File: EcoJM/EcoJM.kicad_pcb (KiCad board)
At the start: 2 copper layers, 49.2 x 99 mm, 50 parts, among them J1 Conn_01x01_Pin, J10 Conn_01x01_Pin, J11 Conn_01x01_Pin, J2 Conn_01x01_Pin, J3 Conn_01x02_Pin, J4 Conn_01x02_Pin, J5 Conn_01x03_Pin, J6 Conn_01x02_Pin, J7 Conn_01x03_Pin, J8 Screw_Terminal_01x02, J9 Screw_Terminal_01x02, Q1 2SD882_C842818, Q2 2SD882_C842818, U1 ACS712xLCTR-30A, U2 MT2492, U3 SIT65HVD230DR, U4 AZ1117-3.3, U5 RS321BXF, U6 STM32F_dev, U7 PC817C_C3025164, U8 PC817C_C3025164

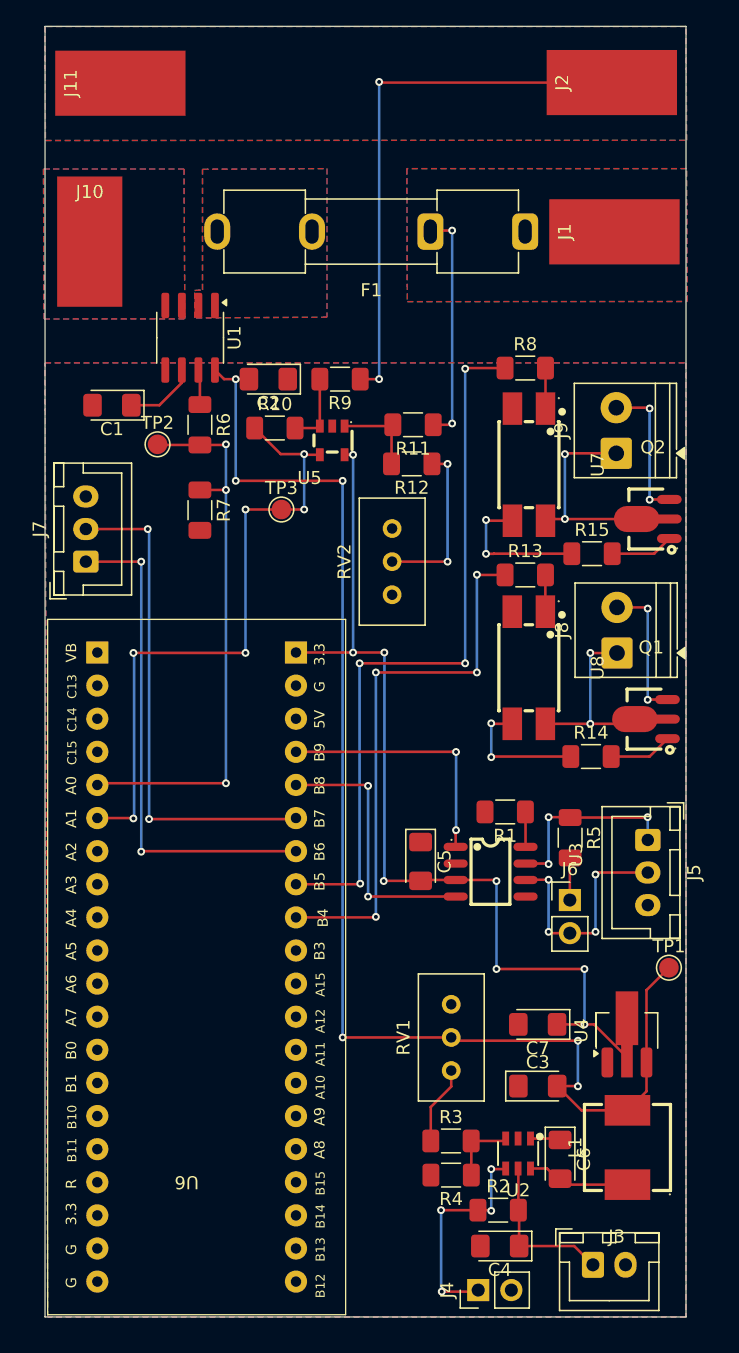
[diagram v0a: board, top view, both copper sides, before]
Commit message: RevA finito, revision, reroute, refurbish
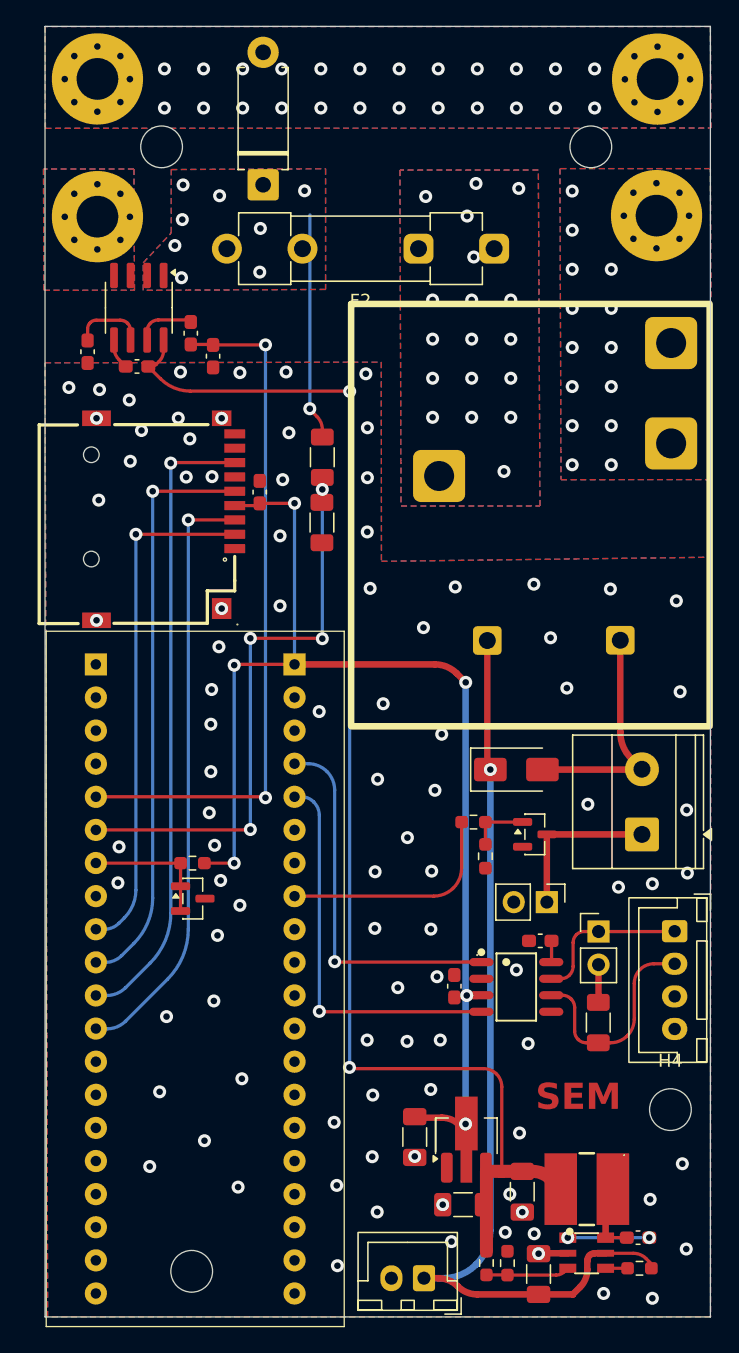
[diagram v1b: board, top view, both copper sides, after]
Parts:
- removed C3, C4: 22u, LED_SMD:LED_1206_3216Metric_Pad1.42x1.75mm_HandSolder
- removed C6: 22n, LED_SMD:LED_1206_3216Metric_Pad1.42x1.75mm_HandSolder
- removed F1: Fuse, Fuse:Fuseholder_Clip-5x20mm_Keystone_3512_Inline_P23.62x7.27mm_D1.02x1.57mm_Horizontal
- removed J11, J2: Conn_01x01_Pin, Connector_Wire:SolderWirePad_1x01_SMD_5x10mm
- removed L1: 10u, EasyEDA:IND-SMD_L7.2-W6.6_GPSR07X0
- removed Q2: 2SD882_C842818, EasyEDA:SOT-89-3_L4.5-W2.5-P1.50-LS4.1-BR
- removed R1, R2, R4: 10k, Resistor_SMD:R_1206_3216Metric_Pad1.30x1.75mm_HandSolder
- removed R13, R8: 470, Resistor_SMD:R_1206_3216Metric_Pad1.30x1.75mm_HandSolder
- removed R14, R15: 100, Resistor_SMD:R_1206_3216Metric_Pad1.30x1.75mm_HandSolder
- removed R3: 68k, Resistor_SMD:R_1206_3216Metric_Pad1.30x1.75mm_HandSolder
- removed R5: 120, Resistor_SMD:R_1206_3216Metric_Pad1.30x1.75mm_HandSolder
- removed RV1, RV2: 10k, Potentiometer_THT:Potentiometer_Bourns_3296W_Vertical
- removed TP1, TP2, TP3: TestPoint, TestPoint:TestPoint_Pad_D1.5mm
- removed U3: SIT65HVD230DR, EasyEDA:SOP-8_L4.9-W3.9-P1.27-LS6.0-BL
- removed U7, U8: PC817C_C3025164, EasyEDA:OPTO-SMD-4_L4.6-W6.5-P2.54-LS10.3-TL
- added C10: 10u, Capacitor_SMD:C_1206_3216Metric_Pad1.33x1.80mm_HandSolder, F.Cu at (103.2, 141.6)
- added C11: 22u, Capacitor_SMD:C_1206_3216Metric_Pad1.33x1.80mm_HandSolder, F.Cu at (97.4, 136.3)
- added C8: 1u, Capacitor_SMD:C_0603_1608Metric_Pad1.08x0.95mm_HandSolder, F.Cu at (81.8, 81.7)
- added C9: 22n, Capacitor_SMD:C_0603_1608Metric_Pad1.08x0.95mm_HandSolder, F.Cu at (110.9, 138.9)
- added C9: 22u, Capacitor_SMD:C_1206_3216Metric_Pad1.33x1.80mm_HandSolder, F.Cu at (102.0, 135.3)
- added D1: P6KE47A, Diode_THT:D_DO-15_P10.16mm_Horizontal, F.Cu at (82.1, 58.1)
- added D2: SS14, Diode_SMD:D_SMA, F.Cu at (101.5, 103.0)
- added F2: Fuse, Fuse:Fuseholder_Clip-5x20mm_Littelfuse_520_Inline_P20.50x5.80mm_D1.30mm_Horizontal, F.Cu at (99.8, 63.0)
- added H1: MountingHole, MountingHole:MountingHole_3.2mm_M3_DIN965, F.Cu at (76.6, 141.4)
- added H2: MountingHole, MountingHole:MountingHole_3.2mm_M3_DIN965, F.Cu at (107.2, 55.2)
- added H3: MountingHole, MountingHole:MountingHole_3.2mm_M3_DIN965, F.Cu at (74.3, 55.2)
- added H4: MountingHole, MountingHole:MountingHole_3.2mm_M3_DIN965, F.Cu at (113.3, 129.0)
- added K1: Relay_SPDT, liblocal:T91 30A, F.Cu at (102.6, 83.4)
- added L2: CD54-6R8M, EasyEDA:IND-SMD_L5.8-W5.2_CD54, F.Cu at (106.9, 135.1)
- added R16: 110k, Resistor_SMD:R_0603_1608Metric_Pad0.98x0.95mm_HandSolder, F.Cu at (99.2, 140.8)
- added R17: 15k, Resistor_SMD:R_0603_1608Metric_Pad0.98x0.95mm_HandSolder, F.Cu at (100.8, 140.8)
- added R18: 10k, Resistor_SMD:R_0603_1608Metric_Pad0.98x0.95mm_HandSolder, F.Cu at (111.0, 141.2)
- added R19: 470, Resistor_SMD:R_0603_1608Metric_Pad0.98x0.95mm_HandSolder, F.Cu at (76.7, 110.1)
- added R20: 2k, Resistor_SMD:R_0603_1608Metric_Pad0.98x0.95mm_HandSolder, F.Cu at (98.2, 107.0)
- added R21: 20k, Resistor_SMD:R_0603_1608Metric_Pad0.98x0.95mm_HandSolder, F.Cu at (99.2, 109.6)
- added U10: MT2492, EasyEDA:SOT-23-6_L2.9-W1.6-P0.95-LS2.8-BL_3, F.Cu at (106.9, 140.1)
- added U9: SIT65HVD230DR, EasyEDA:SOP-8_L4.9-W3.9-P1.27-LS6.0-BL, F.Cu at (101.5, 119.6)
- C1, C2, C5: footprint LED_SMD:LED_1206_3216Metric_Pad1.42x1.75mm_HandSolder -> Capacitor_SMD:C_0603_1608Metric_Pad1.08x0.95mm_HandSolder
- C7: footprint LED_SMD:LED_1206_3216Metric_Pad1.42x1.75mm_HandSolder -> Capacitor_SMD:C_1206_3216Metric_Pad1.33x1.80mm_HandSolder
- J1: value Conn_01x01_Pin -> Screw_Terminal_01x02; footprint Connector_Wire:SolderWirePad_1x01_SMD_5x10mm -> TerminalBlock_Phoenix:TerminalBlock_Phoenix_MKDS-1,5-2_1x02_P5.00mm_Horizontal
- J10: value Conn_01x01_Pin -> Conn_01x02_Pin; footprint Connector_Wire:SolderWirePad_1x01_SMD_5x10mm -> Connector_PinHeader_2.54mm:PinHeader_1x02_P2.54mm_Vertical
- J4: value Conn_01x02_Pin -> Conn_01x04_Pin; footprint Connector_PinHeader_2.54mm:PinHeader_1x02_P2.54mm_Vertical -> Connector_JST:JST_XH_B4B-XH-A_1x04_P2.50mm_Vertical
- J5: value Conn_01x03_Pin -> Conn_01x02_Pin; footprint Connector_JST:JST_XH_B3B-XH-A_1x03_P2.50mm_Vertical -> Connector_PinHeader_2.54mm:PinHeader_1x02_P2.54mm_Vertical
- J6: value Conn_01x02_Pin -> Screw_Terminal_01x01; footprint Connector_PinHeader_2.54mm:PinHeader_1x02_P2.54mm_Vertical -> Libmain:M3_PCONN_1x01
- J7: value Conn_01x03_Pin -> Screw_Terminal_01x01; footprint Connector_JST:JST_XH_B3B-XH-A_1x03_P2.50mm_Vertical -> Libmain:M3_PCONN_1x01
- J8, J9: value Screw_Terminal_01x02 -> Screw_Terminal_01x01; footprint TerminalBlock_Phoenix:TerminalBlock_Phoenix_PT-1,5-2-3.5-H_1x02_P3.50mm_Horizontal -> Libmain:M3_PCONN_1x01
- Q1: value 2SD882_C842818 -> AO3400A; footprint EasyEDA:SOT-89-3_L4.5-W2.5-P1.50-LS4.1-BR -> Package_TO_SOT_SMD:SOT-23
- R10: value 2.2k -> 2.7k
- R11: value 47k -> 10k; footprint Resistor_SMD:R_1206_3216Metric_Pad1.30x1.75mm_HandSolder -> Capacitor_SMD:C_0603_1608Metric_Pad1.08x0.95mm_HandSolder
- R12: value 2.2k -> 120
- R6, R7: footprint Resistor_SMD:R_1206_3216Metric_Pad1.30x1.75mm_HandSolder -> Capacitor_SMD:C_0603_1608Metric_Pad1.08x0.95mm_HandSolder
- U2: value MT2492 -> TL431DBZ; footprint EasyEDA:SOT-23-6_L2.9-W1.6-P0.95-LS2.8-BL_3 -> Package_TO_SOT_SMD:SOT-23
- U5: value RS321BXF -> HX TF PUSH; footprint EasyEDA:SOT-23-5_L2.9-W1.6-P0.95-LS2.8-BL -> EasyEDA:TF-SMD_TF-PUSH
- moved J10 61.6 mm to (103.9, 113.1), turned to -90 degrees
- moved J7 57.4 mm to (112.3, 50.0), turned to 0 degrees
- moved J6 52.9 mm to (112.2, 60.4)
- moved J8 52.1 mm to (69.4, 60.5), turned to 0 degrees
- moved J9 49.1 mm to (69.4, 50.0), turned to 0 degrees
- moved J1 46.3 mm to (111.2, 107.9)
- moved R12 45.2 mm to (107.8, 122.4), turned to 90 degrees
- moved R11 40.8 mm to (103.4, 116.1), turned to 0 degrees
- moved U2 31.7 mm to (76.7, 112.8), turned to 0 degrees
- moved J4 31.4 mm to (113.7, 115.3), turned to -90 degrees
- moved U4 14.7 mm to (97.7, 131.0)
- moved U5 14.1 mm to (74.6, 83.8), turned to -90 degrees
- moved J3 13.0 mm to (94.4, 142.0), turned to 180 degrees
- moved C7 12.8 mm to (93.7, 131.1), turned to -90 degrees
- moved Q1 12.6 mm to (102.9, 107.9)
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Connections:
- C5 pad 1: GND -> +3.3V
- C5 pad 2: +3.3V -> GND
- J1 pad 1: /VDCH+_IN -> Net-(J1-Pin_1)
- J10 pad 1: /VDCH+_OUT -> Net-(J1-Pin_1)
- J4 pad 1: Net-(J4-Pin_1) -> /CANH
- J4 pad 2: GND -> /CANL
- J5 pad 1: /CAN_H -> /CANH
- J5 pad 2: /CAN_L -> Net-(J5-Pin_2)
- J6 pad 1: Net-(J6-Pin_1) -> /VDCH+_IN
- J7 pad 1: /UART_TX -> /VDCH-
- J8 pad 1: Net-(J8-Pin_1) -> /VDCH+_OUT
- J9 pad 1: Net-(J9-Pin_1) -> /VDCH-
- Q1 pad 2: Net-(J8-Pin_1) -> GND
- Q1 pad 3: Net-(J8-Pin_2) -> Net-(J1-Pin_1)
- R10 pad 2: Net-(U5--IN) -> GND
- R11 pad 1: /VDCH+_IN -> GND
- R11 pad 2: Net-(U5-+IN) -> Net-(U9-RS)
- R12 pad 1: Net-(R12-Pad1) -> /CANL
- R12 pad 2: Net-(U5-+IN) -> Net-(J5-Pin_2)
- R9 pad 1: /VDCH- -> /Voltage_M
- R9 pad 2: Net-(U5--IN) -> /VDCH+_INFUSED
- U1 pad 1: Net-(F1-Pad2) -> /VDCH+_INFUSED
- U1 pad 2: Net-(F1-Pad2) -> /VDCH+_INFUSED
- U2 pad 1: Net-(U2-BS) -> /VREF
- U2 pad 2: GND -> /VREF
- U2 pad 3: Net-(U2-FB) -> GND
- U5 pad 1: Net-(U5-+IN) -> unconnected-(U5-DAT2-Pad1)
- U5 pad 2: GND -> /SD_CS
- U5 pad 3: Net-(U5--IN) -> /SPI_MOSI
- U5 pad 4: /Voltage_M -> +3.3V
- U5 pad 5: +3.3V -> /SPI_SCK
- U6 pad 12: /SSR1 -> unconnected-(U6-B4-Pad12)
- U6 pad 14: /UART_TX -> unconnected-(U6-B6-Pad14)
- U6 pad 15: /UART_RX -> unconnected-(U6-B7-Pad15)
- U6 pad 29: unconnected-(U6-A7-Pad29) -> /SPI_MOSI
- U6 pad 30: unconnected-(U6-A6-Pad30) -> /SPI_MISO
- U6 pad 31: unconnected-(U6-A5-Pad31) -> /SPI_SCK
- U6 pad 32: unconnected-(U6-A4-Pad32) -> /SD_CS
- U6 pad 34: unconnected-(U6-A2-Pad34) -> /VREF
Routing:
- net +12V: track 12.2 -> 73.0 mm, vias 0 -> 1
- net /SPI_MISO: track 0.00 -> 48.8 mm, vias 0 -> 1
- net /SPI_MOSI: track 0.00 -> 46.2 mm, vias 0 -> 1
- net /SPI_SCK: track 0.00 -> 44.8 mm, vias 0 -> 1
- net /SSR1: track 42.3 -> 0.00 mm, vias 4 -> 0
- net /VDCH-: track 42.1 -> 0.00 mm, vias 2 -> 24
- net /SD_CS: track 0.00 -> 39.7 mm, vias 0 -> 1
- net /UART_TX: track 38.4 -> 0.00 mm, vias 2 -> 0
- net /UART_RX: track 38.3 -> 0.00 mm, vias 2 -> 0
- net /SSR0: track 55.7 -> 17.6 mm, vias 4 -> 0
- net +3.3V: track 73.5 -> 96.5 mm, vias 8 -> 6
- net /CAN_L: track 18.1 -> 0.00 mm, vias 4 -> 0
- net Net-(D2-A): track 0.00 -> 18.1 mm
- net /VDCH+_IN: track 18.0 -> 0.00 mm, vias 2 -> 14
- net /VDCH+_INFUSED: track 0.00 -> 17.4 mm, vias 0 -> 9
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- added copper zone on B.Cu, net /VDCH+_INFUSED
- added copper zone on F.Cu, net /VDCH+_INFUSED
- added copper zone on B.Cu, net /VDCH+_INSW
- added copper zone on F.Cu, net /VDCH+_INSW
- removed copper zone on B.Cu, net Net-(F1-Pad2)
- removed copper zone on F.Cu, net Net-(F1-Pad2)
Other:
- board size 49.2 x 99 mm -> 51 x 99 mm
- board text added: "SEM"
